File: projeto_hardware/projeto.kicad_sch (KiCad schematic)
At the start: 95 parts, among them J1 arrego, J2 arrego, J3 Conn_01x10_Pin, J4 arrego, J5 arrego, P1 Card_SD, Q1 BC847, Q2 BC847, SW1 BOOT, SW2 BTN2, SW3 RST, SW5 BTN1, SW6 SW_DPDT_x2, U1 ESP32-S3-WROOM-1, U10 AP63203WU, U11 CD4051B, U2 QRE1113, U3 QRE1113, U4 ICM-42688, U5 DRV825, U6 DRV825, U7 QRE1113, U8 QRE1113, U9 LM358, con1 BATERIA

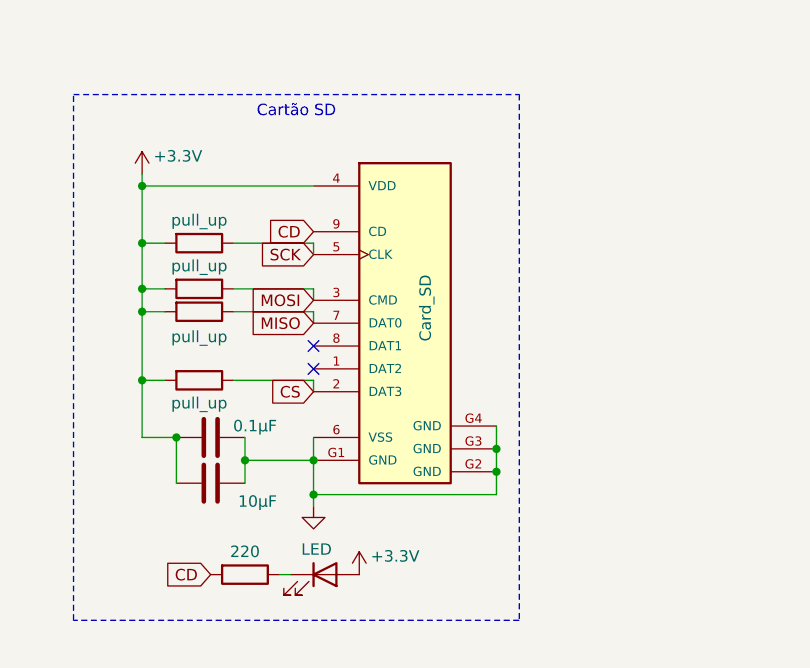
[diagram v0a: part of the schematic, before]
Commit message: projeto step
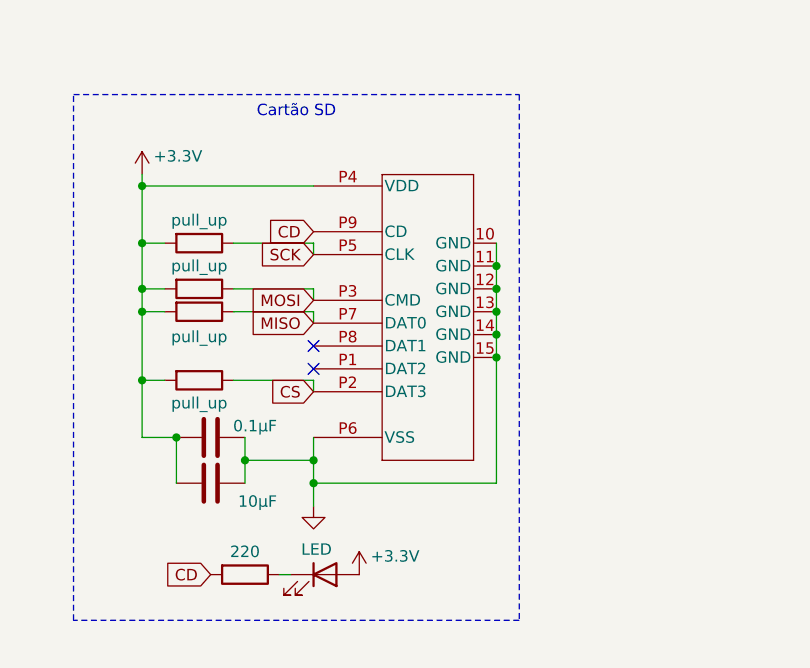
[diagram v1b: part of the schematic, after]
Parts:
- removed P1: Card_SD, Library:Micro_SD_card, symbol ST-TF-003A:ST-TF-003A
- added J6: MEM2075-00-140-01-A, Library:MEM2075-00-140-01-A_GCT, symbol 2026-03-26_23-56-39:MEM2075-00-140-01-A
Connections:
- net +3.3V: now also J6.P4 (VDD)
- net CD: now also J6.P9 (CD)
- net CS: now also J6.P2 (DAT3)
- net GND: now also J6.10 (GND), J6.11 (GND), J6.12 (GND), J6.13 (GND), J6.14 (GND), J6.15 (GND), J6.P6 (VSS)
- net MISO: now also J6.P7 (DAT0)
- net MOSI: now also J6.P3 (CMD)
- net SCK: now also J6.P5 (CLK)
